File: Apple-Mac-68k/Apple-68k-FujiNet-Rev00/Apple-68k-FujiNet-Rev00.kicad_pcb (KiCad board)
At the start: 2 copper layers, 80.8 x 70.6 mm, 28 parts, among them J1 Apple IDC-20, J2 Logic Analyzer, J3 UART, J4 SWD, P1 ST-TF-003A, SW1 ButtonA, SW2 Safe Reset, U1 Pico, U2 ESP32-S3-DevKitC-1 N16R8

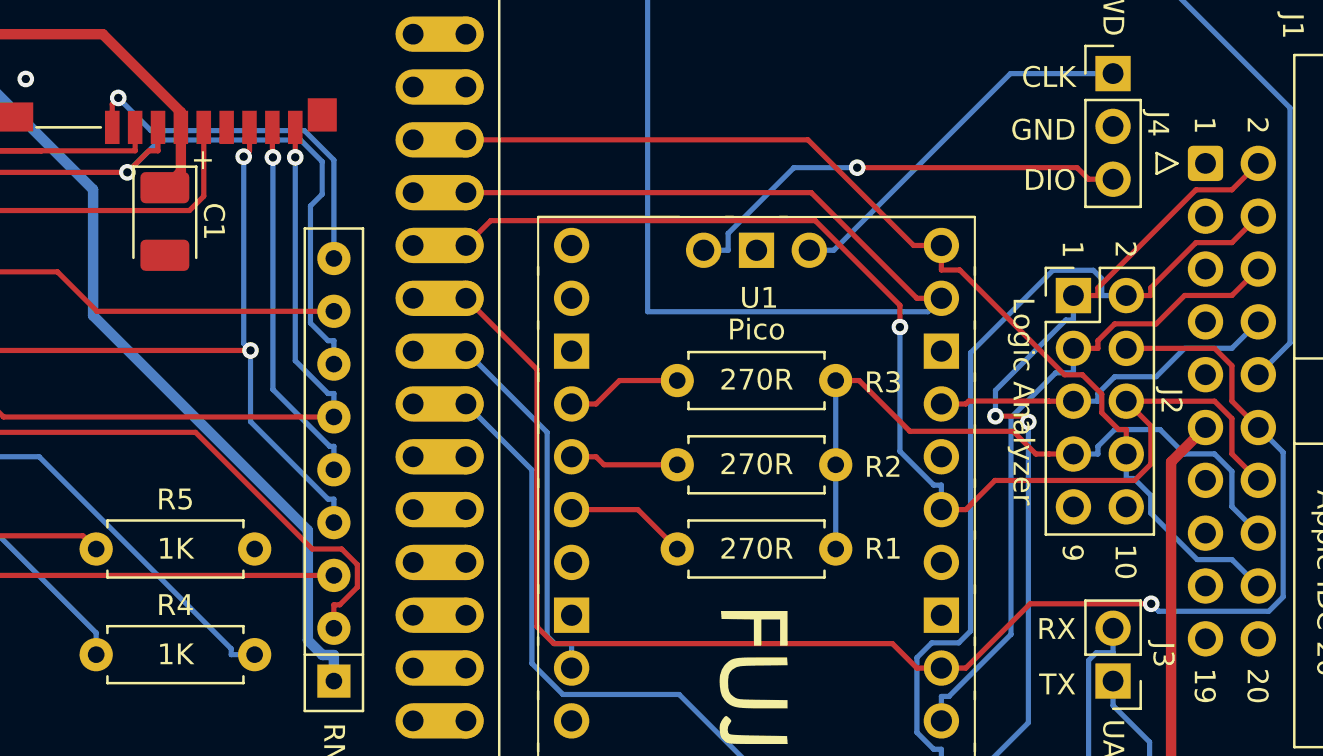
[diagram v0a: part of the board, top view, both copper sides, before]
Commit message: fix routes
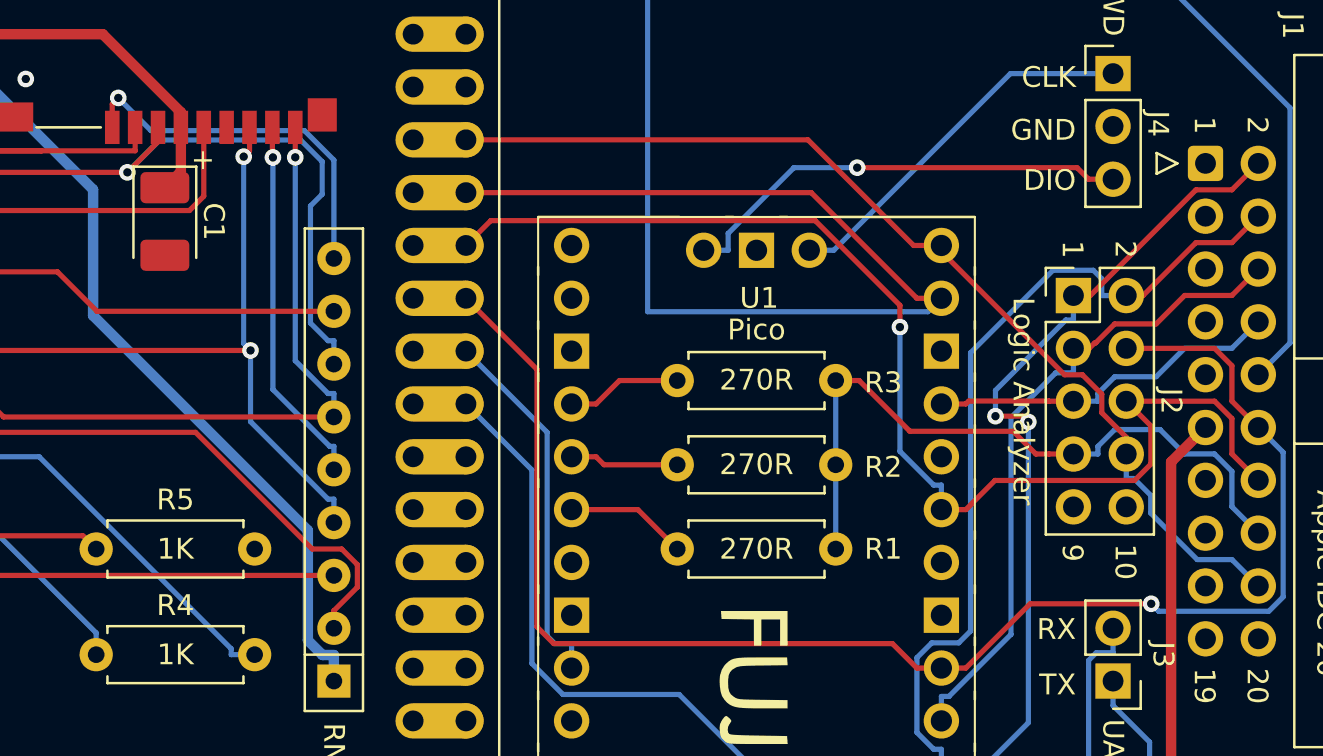
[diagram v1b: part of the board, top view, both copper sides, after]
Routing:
- net /WR_DATA: track 52.6 -> 51.9 mm
